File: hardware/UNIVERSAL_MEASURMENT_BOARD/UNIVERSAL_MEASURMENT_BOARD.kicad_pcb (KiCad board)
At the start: 2 copper layers, 180 parts, among them J1 2606-1110_010-000, J2 2606-1110_010-000, J28 FTSH-107-01-L-D-K, J3 2606-1110_010-000, J4 2606-1110_010-000, J5 2604-1104, U1 ADS8863IDGS, U10 TPS54202HDDCR, U11 CD4097BM, U12 TPS54202HDDCR, U13 L7805ABD2T-TR, U14 ADM3055EBRIZ-RL, U15 TLV76133KVUR, U16 TLV76133KVUR, U17 ESDS304DBVR, U18 ESDS304DBVR, U2 LT3471EDD#PBF, U3 MAX6063AEUR+T, U4 PGA280AIPW, U5 ISL21010CFH315Z-TK, U6 STM32G484RET3, U7 L7812ABD2T-TR, U8 MC7815BDTRKG, U9 MC79M15CDTRKG, Y1 ECS-1612MV

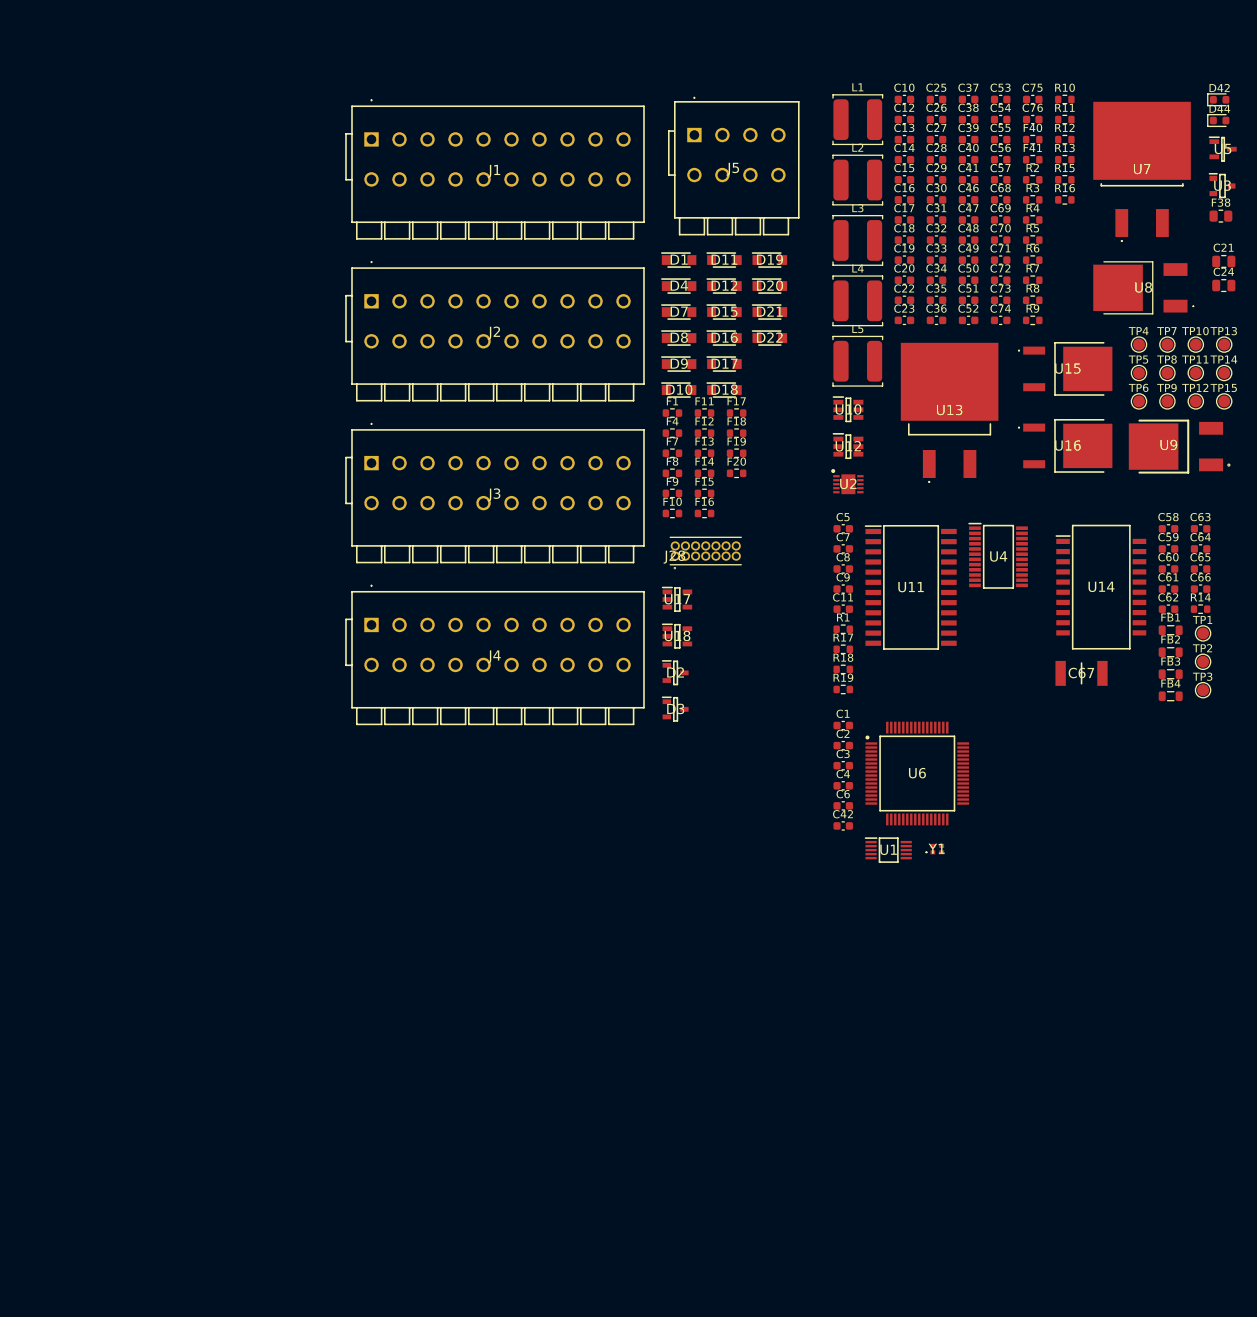
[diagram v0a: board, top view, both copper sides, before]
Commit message: first outcom of pcb design
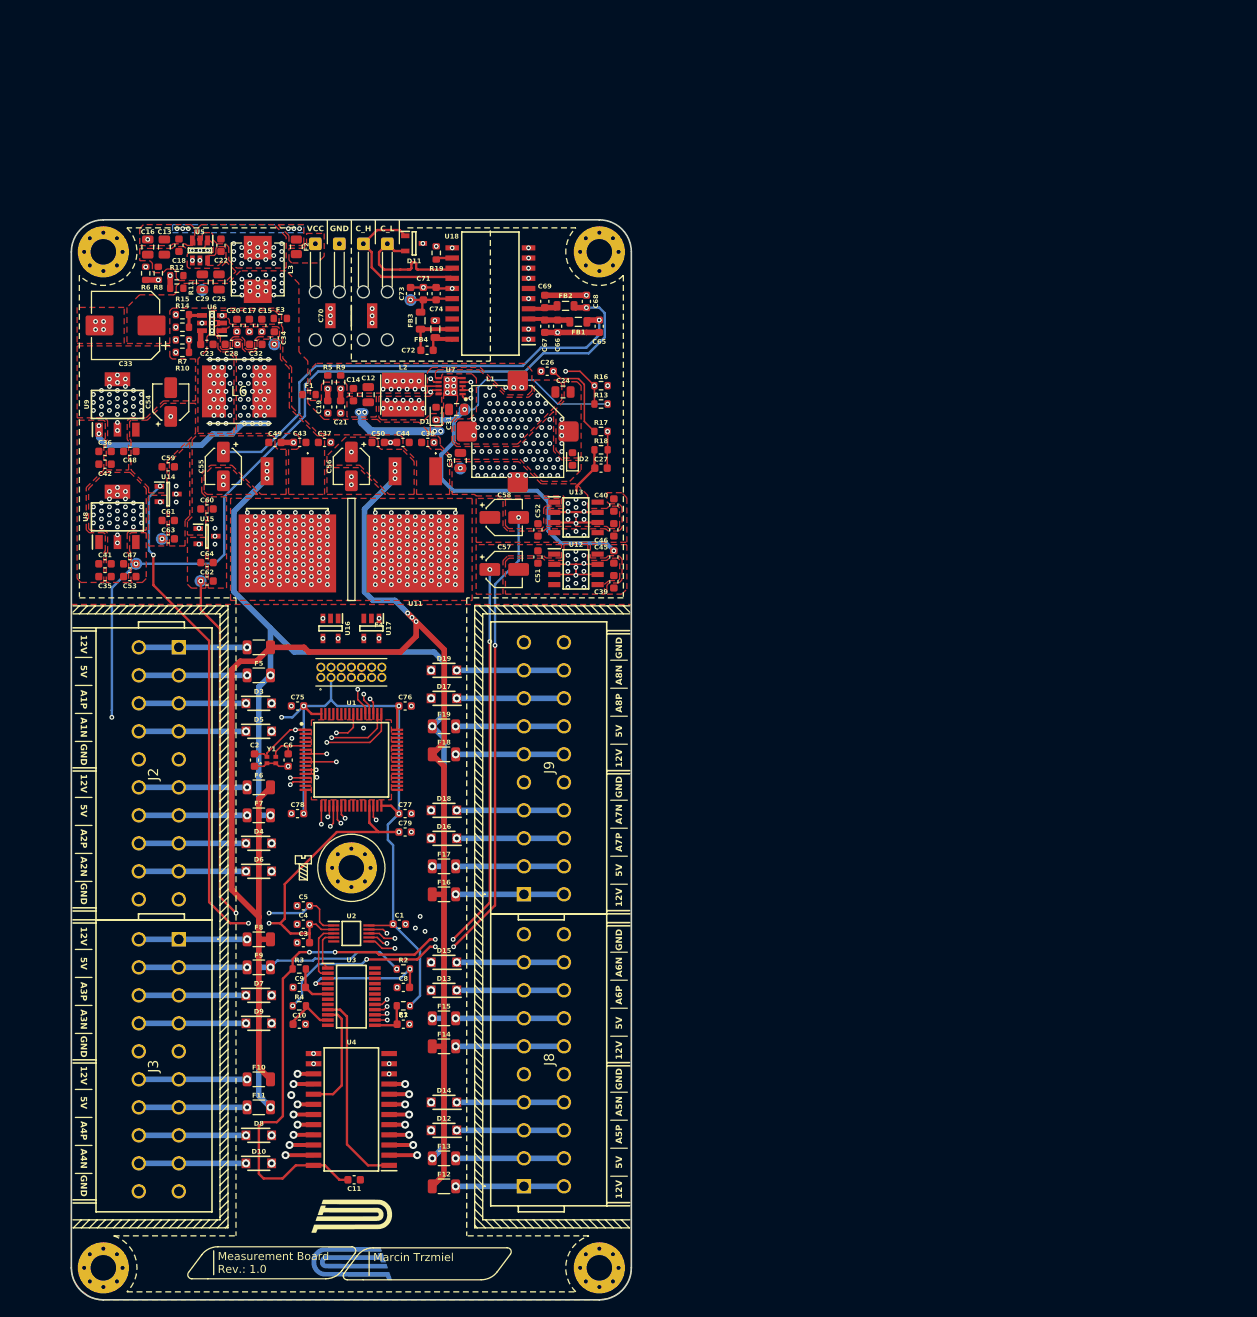
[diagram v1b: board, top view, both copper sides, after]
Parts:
- removed D20, D21, D22: ATV02W150-HF, ATV02W150-HF:SODFL3718X130N
- removed D42, D44: CDBU0340, Diode_SMD:D_0603_1608Metric
- removed F20: 100mA, Resistor_SMD:R_0603_1608Metric
- removed F38: 1,5A, Resistor_SMD:R_0805_2012Metric
- removed F40, F41: 300mA, Resistor_SMD:R_0603_1608Metric
- removed J28: FTSH-107-01-L-D-K, FTSH-107-01-L-D-K:FTSH-107-XX-YYY-D-K
- removed L4: 10uH, Inductor_SMD:L_TDK_VLS6045EX_VLS6045AF
- removed L5: 15uH, Inductor_SMD:L_TDK_VLS6045EX_VLS6045AF
- removed TP13: 3V3, TestPoint:TestPoint_Pad_D1.5mm
- removed TP14: 3V0A, TestPoint:TestPoint_Pad_D1.5mm
- removed the U4 at (182.1, 104.9)
- added C43: 330nF, REST:C_0603_1608Metric, F.Cu at (94.8, 90.6)
- added C44: 330nF, REST:C_0603_1608Metric, F.Cu at (107.7, 90.6)
- added C45: 330nF, REST:C_0603_1608Metric, F.Cu at (134.0, 104.9)
- added C77: 100nF, REST:C_0603_1608Metric, F.Cu at (107.9, 137.0)
- added C78: 100nF, REST:C_0603_1608Metric, F.Cu at (94.5, 137.0)
- added C79: 100nF, REST:C_0603_1608Metric, F.Cu at (107.9, 139.3)
- added D13: ATV02W150-HF, ATV02W150-HF:SODFL3718X130N, F.Cu at (112.8, 159.1)
- added D14: ATV02W150-HF, ATV02W150-HF:SODFL3718X130N, F.Cu at (112.8, 173.1)
- added D5: ATV02W150-HF, ATV02W150-HF:SODFL3718X130N, F.Cu at (89.7, 126.7)
- added D6: ATV02W150-HF, ATV02W150-HF:SODFL3718X130N, F.Cu at (89.7, 144.2)
- added F2: 1,5A, REST:F_0805_2012Metric, F.Cu at (94.3, 66.1)
- added F3: 300mA, REST:F_0603_1608Metric, F.Cu at (92.3, 75.1)
- added F5: 100mA, REST:F_1206_3216Metric, F.Cu at (89.7, 119.7)
- added F6: 100mA, REST:F_1206_3216Metric, F.Cu at (89.7, 133.7)
- added J6: Conn_01x01_Socket, REST:SolderWire-0.1sqmm_1x01_D0.4mm_OD1mm_Relief2x, F.Cu at (105.7, 65.8)
- added J7: Conn_01x01_Socket, REST:SolderWire-0.1sqmm_1x01_D0.4mm_OD1mm_Relief2x, F.Cu at (99.7, 65.8)
- added J8: 2606-1110_010-000, 2601-1110:26011110, F.Cu at (125.9, 167.7)
- added J9: 2606-1110_010-000, 2601-1110:26011110, F.Cu at (125.9, 131.2)
- added L6: ASPIAIG-S8050-221M-T, ASPIAIG-S8050-221M-T:INDPM8080X520N, F.Cu at (87.2, 84.2)
- added REF**: MountingHole_3.2mm_M3_Pad_Via, REST:MountingHole_3.2mm_M3_Pad_Via, F.Cu at (132.2, 193.8)
- added REF**: Screw_Generic_2.0x3.0mm_SilkScreen, Symbol:Screw_Generic_2.0x3.0mm_SilkScreen, F.Cu at (95.2, 143.8)
- added REF**: MountingHole_3.2mm_M3_Pad_Via, REST:MountingHole_3.2mm_M3_Pad_Via, F.Cu at (132.2, 66.8)
- added REF**: MountingHole_3.2mm_M3_Pad_Via, REST:MountingHole_3.2mm_M3_Pad_Via, F.Cu at (101.2, 143.8)
- added REF**: MountingHole_3.2mm_M3_Pad_Via, REST:MountingHole_3.2mm_M3_Pad_Via, F.Cu at (70.2, 193.8)
- added REF**: MountingHole_3.2mm_M3_Pad_Via, REST:MountingHole_3.2mm_M3_Pad_Via, F.Cu at (70.2, 66.8)
- added U11: L7812ABD2T-TR, L7812ABD2T-TR:L7812ABD2TTR, F.Cu at (109.2, 99.6)
- C1, C11, C19, C2, C22, C32, C38, C40, C49, C5, C6, C62, C75, C8, C9: footprint Capacitor_SMD:C_0603_1608Metric -> REST:C_0603_1608Metric
- C10: value 220uF -> 470nF; footprint Capacitor_SMD:C_0603_1608Metric -> REST:C_0603_1608Metric
- C12: value 1uF -> 10uF; footprint Capacitor_SMD:C_0603_1608Metric -> REST:C_0805_2012Metric
- C13: value 100nF -> 22uF; footprint Capacitor_SMD:C_0603_1608Metric -> REST:C_0805_2012Metric
- C14, C26, C47, C48, C50, C73, C76: value 22uF -> 100nF; footprint Capacitor_SMD:C_0603_1608Metric -> REST:C_0603_1608Metric
- C15: value 330nF -> 22uF; footprint Capacitor_SMD:C_0603_1608Metric -> REST:C_0603_1608Metric
- C16: value 220nF -> 22uF; footprint Capacitor_SMD:C_0603_1608Metric -> REST:C_0805_2012Metric
- C17, C35, C36, C39: value 1uF -> 22uF; footprint Capacitor_SMD:C_0603_1608Metric -> REST:C_0603_1608Metric
- C18, C68: value 10uF -> 100nF; footprint Capacitor_SMD:C_0603_1608Metric -> REST:C_0603_1608Metric
- C20, C23: value 1uF -> 100nF; footprint Capacitor_SMD:C_0603_1608Metric -> REST:C_0603_1608Metric
- C21: value 4.7uF -> 1uF; footprint Capacitor_SMD:C_0805_2012Metric -> REST:C_0603_1608Metric
- C24: value 10uF -> 1uF; footprint Capacitor_SMD:C_0805_2012Metric -> REST:C_0805_2012Metric
- C25: value 75pF -> 22uF; footprint Capacitor_SMD:C_0603_1608Metric -> REST:C_0805_2012Metric
- C27: value 330nF -> 75pF; footprint Capacitor_SMD:C_0603_1608Metric -> REST:C_0603_1608Metric
- C28: value 220nF -> 100nF; footprint Capacitor_SMD:C_0603_1608Metric -> REST:C_0603_1608Metric
- C29: value 1uF -> 22uF; footprint Capacitor_SMD:C_0603_1608Metric -> REST:C_0805_2012Metric
- C3: value 10nF -> 100nF; footprint Capacitor_SMD:C_0603_1608Metric -> REST:C_0603_1608Metric
- C30: value 100nF -> 10uF; footprint Capacitor_SMD:C_0603_1608Metric -> REST:C_0805_2012Metric
- C31: value 22uF -> 4.7uF; footprint Capacitor_SMD:C_0603_1608Metric -> REST:C_0805_2012Metric
- C33: value 100nF -> 220uF; footprint Capacitor_SMD:C_0603_1608Metric -> REST:CP_Elec_8x10
- C34, C37, C53: value 100nF -> 22uF; footprint Capacitor_SMD:C_0603_1608Metric -> REST:C_0603_1608Metric
- C4, C71: value 100nF -> 10nF; footprint Capacitor_SMD:C_0603_1608Metric -> REST:C_0603_1608Metric
- C41: value 22uF -> 330nF; footprint Capacitor_SMD:C_0603_1608Metric -> REST:C_0603_1608Metric
- C42, C46: value 100nF -> 330nF; footprint Capacitor_SMD:C_0603_1608Metric -> REST:C_0603_1608Metric
- C51: value 22uF -> 220nF; footprint Capacitor_SMD:C_0603_1608Metric -> REST:C_0603_1608Metric
- C52: value 330nF -> 220nF; footprint Capacitor_SMD:C_0603_1608Metric -> REST:C_0603_1608Metric
- C54: footprint Capacitor_SMD:C_0603_1608Metric -> REST:CP_Elec_4x5.8
- C55: value 22uF -> 10uF; footprint Capacitor_SMD:C_0603_1608Metric -> REST:CP_Elec_4x5.8
- C56: value 330nF -> 10uF; footprint Capacitor_SMD:C_0603_1608Metric -> REST:CP_Elec_4x5.8
- C57: value 100nF -> 1uF; footprint Capacitor_SMD:C_0603_1608Metric -> REST:CP_Elec_4x5.4
- C58: value 47uF -> 1uF; footprint Capacitor_SMD:C_0603_1608Metric -> REST:CP_Elec_4x5.4
- C59, C60: value 47uF -> 1uF; footprint Capacitor_SMD:C_0603_1608Metric -> REST:C_0603_1608Metric
- C61: value 47uF -> 100nF; footprint Capacitor_SMD:C_0603_1608Metric -> REST:C_0603_1608Metric
- C63: value 100nF -> 1uF; footprint Capacitor_SMD:C_0603_1608Metric -> REST:C_0603_1608Metric
- C64: value 10nF -> 1uF; footprint Capacitor_SMD:C_0603_1608Metric -> REST:C_0603_1608Metric
- C65: value 10nF -> 47uF; footprint Capacitor_SMD:C_0603_1608Metric -> REST:C_0603_1608Metric
- C66: value 100nF -> 47uF; footprint Capacitor_SMD:C_0603_1608Metric -> REST:C_0603_1608Metric
- C67: value 4.7nF/Y2 -> 100nF; footprint S252B222K502CT:CAPC5728X280N -> REST:C_0603_1608Metric
- C69: value 22uF -> 10nF; footprint Capacitor_SMD:C_0603_1608Metric -> REST:C_0603_1608Metric
- C7: value 470nF -> 100nF; footprint Capacitor_SMD:C_0603_1608Metric -> REST:C_0603_1608Metric
- C70: value 330nF -> 4.7nF/Y2; footprint Capacitor_SMD:C_0603_1608Metric -> S252B222K502CT:CAPC5728X280N
- C72: value 10uF -> 47uF; footprint Capacitor_SMD:C_0603_1608Metric -> REST:C_0603_1608Metric
- C74: value 330nF -> 47uF; footprint Capacitor_SMD:C_0603_1608Metric -> REST:C_0603_1608Metric
- D1: value ATV02W150-HF -> CDBU0340; footprint ATV02W150-HF:SODFL3718X130N -> REST:D_0603_1608Metric
- D11: value ATV02W150-HF -> PESD5V0L2BT,215; footprint ATV02W150-HF:SODFL3718X130N -> PESD5V0L2BT,215:SOT95P230X110-3N
- D2: value PESD5V0L2BT,215 -> CDBU0340; footprint PESD5V0L2BT,215:SOT95P230X110-3N -> REST:D_0603_1608Metric
- D3: value PESD5V0L2BT,215 -> ATV02W150-HF; footprint PESD5V0L2BT,215:SOT95P230X110-3N -> ATV02W150-HF:SODFL3718X130N
- F1: value 100mA -> 300mA; footprint Resistor_SMD:R_0603_1608Metric -> REST:F_0603_1608Metric
- F10, F11, F12, F13, F14, F15, F16, F17, F18, F19, F4, F7, F8, F9: footprint Resistor_SMD:R_0603_1608Metric -> REST:F_1206_3216Metric
- FB1, FB2, FB3, FB4: footprint Inductor_SMD:L_0805_2012Metric -> REST:L_0805_2012Metric
- J1: value 2606-1110_010-000 -> FTSH-107-01-L-D-K; footprint 2601-1110:26011110 -> FTSH-107-01-L-D-K:FTSH-107-XX-YYY-D-K
- J4: value 2606-1110_010-000 -> Conn_01x01_Socket; footprint 2601-1110:26011110 -> REST:SolderWire-0.1sqmm_1x01_D0.4mm_OD1mm_Relief2x
- J5: value 2604-1104 -> Conn_01x01_Socket; footprint 2601-1104:26011104 -> REST:SolderWire-0.1sqmm_1x01_D0.4mm_OD1mm_Relief2x
- L1: value 2.2uH -> PM3604-5-RC; footprint Inductor_SMD:L_TDK_VLS6045EX_VLS6045AF -> PM3604-5-RC:PM3604-5-RC
- L2: value 68uH/1.4A -> 74408943100; footprint Inductor_SMD:L_TDK_VLS6045EX_VLS6045AF -> 74408943100:WE-SPC_48XX78
- L3: value 68uH/1.4A -> 74437349560; footprint Inductor_SMD:L_TDK_VLS6045EX_VLS6045AF -> 74437349560:74437349560
- R1: value 22R -> 10R; footprint Resistor_SMD:R_0603_1608Metric -> REST:R_0603_1608Metric
- R10: value 649kR -> 73.2kR; footprint Resistor_SMD:R_0603_1608Metric -> REST:R_0603_1608Metric
- R11: footprint Resistor_SMD:R_0603_1608Metric -> REST:R_0603_1608Metric
- R12: value 64.9kR -> 10kR; footprint Resistor_SMD:R_0603_1608Metric -> REST:R_0603_1608Metric
- R13: value 10kR -> 255kR; footprint Resistor_SMD:R_0603_1608Metric -> REST:R_0603_1608Metric
- R14: value 100kR -> -R; footprint Resistor_SMD:R_0603_1608Metric -> REST:R_0603_1608Metric
- R15: value 15kR -> -R; footprint Resistor_SMD:R_0603_1608Metric -> REST:R_0603_1608Metric
- R16: value 274kR -> 15kR; footprint Resistor_SMD:R_0603_1608Metric -> REST:R_0603_1608Metric
- R17: value 22R -> 15kR; footprint Resistor_SMD:R_0603_1608Metric -> REST:R_0603_1608Metric
- R18: value 10R -> 274kR; footprint Resistor_SMD:R_0603_1608Metric -> REST:R_0603_1608Metric
- R19: value 10R -> 100kR; footprint Resistor_SMD:R_0603_1608Metric -> REST:R_0603_1608Metric
- R2: value 11kR -> 10R; footprint Resistor_SMD:R_0603_1608Metric -> REST:R_0603_1608Metric
- R3: value 11kR -> 22R; footprint Resistor_SMD:R_0603_1608Metric -> REST:R_0603_1608Metric
- R4: value 255kR -> 22R; footprint Resistor_SMD:R_0603_1608Metric -> REST:R_0603_1608Metric
- R5: value 15kR -> 11kR; footprint Resistor_SMD:R_0603_1608Metric -> REST:R_0603_1608Metric
- R6: value 681kR -> 649kR; footprint Resistor_SMD:R_0603_1608Metric -> REST:R_0603_1608Metric
- R7: value -R -> 681kR; footprint Resistor_SMD:R_0603_1608Metric -> REST:R_0603_1608Metric
- R8: value 73.2kR -> 64.9kR; footprint Resistor_SMD:R_0603_1608Metric -> REST:R_0603_1608Metric
- R9: value -R -> 11kR; footprint Resistor_SMD:R_0603_1608Metric -> REST:R_0603_1608Metric
- TP1: value C5V -> M15V; footprint TestPoint:TestPoint_Pad_D1.5mm -> REST:TestPoint_Pad_D1.5mm; moved to B.Cu
- TP10: value 12VA -> -15VA; footprint TestPoint:TestPoint_Pad_D1.5mm -> REST:TestPoint_Pad_D1.5mm; moved to B.Cu
- TP11: value 5VA -> 1V5A; footprint TestPoint:TestPoint_Pad_D1.5mm -> REST:TestPoint_Pad_D1.5mm; moved to B.Cu
- TP12: value 3V3A -> 3V0A; footprint TestPoint:TestPoint_Pad_D1.5mm -> REST:TestPoint_Pad_D1.5mm; moved to B.Cu
- TP15: value 1V5A -> CVISO; footprint TestPoint:TestPoint_Pad_D1.5mm -> REST:TestPoint_Pad_D1.5mm; moved to B.Cu
- TP2: value C3V -> -18V; footprint TestPoint:TestPoint_Pad_D1.5mm -> REST:TestPoint_Pad_D1.5mm; moved to B.Cu
- TP3: value CVISO -> 7V; footprint TestPoint:TestPoint_Pad_D1.5mm -> REST:TestPoint_Pad_D1.5mm; moved to B.Cu
- TP4: value M15V -> 18V; footprint TestPoint:TestPoint_Pad_D1.5mm -> REST:TestPoint_Pad_D1.5mm; moved to B.Cu
- TP5: value 18V -> 3V3; footprint TestPoint:TestPoint_Pad_D1.5mm -> REST:TestPoint_Pad_D1.5mm; moved to B.Cu
- TP6: value -18V -> 3V3A; footprint TestPoint:TestPoint_Pad_D1.5mm -> REST:TestPoint_Pad_D1.5mm; moved to B.Cu
- TP7: value 7V -> 5VA; footprint TestPoint:TestPoint_Pad_D1.5mm -> REST:TestPoint_Pad_D1.5mm; moved to B.Cu
- TP8: value 15VA -> 12VA; footprint TestPoint:TestPoint_Pad_D1.5mm -> REST:TestPoint_Pad_D1.5mm; moved to B.Cu
- TP9: value -15VA -> 15VA; footprint TestPoint:TestPoint_Pad_D1.5mm -> REST:TestPoint_Pad_D1.5mm; moved to B.Cu
- U1: value ADS8863IDGS -> STM32G484RET3; footprint ADS8863IDGS:SOP50P490X110-10N -> STM32G484RET3:QFP50P1200X1200X160-64N
- U10: value TPS54202HDDCR -> L7805ABD2T-TR; footprint TPS54202HDDCR:SOT95P280X110-6N -> L7805ABD2T-TR:L7805ABD2TTR
- U12: value TPS54202HDDCR -> L78L15ACD13TR; footprint TPS54202HDDCR:SOT95P280X110-6N -> LP358DR:SOIC127P600X175-8N
- U13: value L7805ABD2T-TR -> L79L15ACD13TR; footprint L7805ABD2T-TR:L7805ABD2TTR -> LP358DR:SOIC127P600X175-8N
- U14: value ADM3055EBRIZ-RL -> ISL21010CFH315Z-TK; footprint ADM3055EBRIZ-RL:SOIC127P1030X264-20N -> ISL21010CFH315Z-TK:SOT95P237X112-3N
- U15: value TLV76133KVUR -> ISL21010CFH330Z-TK; footprint TLV76133KVUR:TLV76133KVUR -> ISL21010CFH315Z-TK:SOT95P237X112-3N
- U16: value TLV76133KVUR -> ESDS304DBVR; footprint TLV76133KVUR:TLV76133KVUR -> ESDS304DBVR:SOT95P280X145-5N
- U18: value ESDS304DBVR -> ADM3055EBRIZ-RL; footprint ESDS304DBVR:SOT95P280X145-5N -> ADM3055EBRIZ-RL:SOIC127P1030X264-20N
- U2: value LT3471EDD#PBF -> ADS8863IDGS; footprint LT3471EDD#PBF:SON50P300X300X80-11N-D -> ADS8863IDGS:SOP50P490X110-10N
- U3: value MAX6063AEUR+T -> PGA280AIPW; footprint MAX6063AEUR+T:SOT95P229X119-3N -> PGA280AIPW:SOP65P640X120-24N
- U5: value ISL21010CFH315Z-TK -> TPS54202HDDCR; footprint ISL21010CFH315Z-TK:SOT95P237X112-3N -> TPS54202HDDCR:SOT95P280X110-6N
- U6: value STM32G484RET3 -> TPS54202HDDCR; footprint STM32G484RET3:QFP50P1200X1200X160-64N -> TPS54202HDDCR:SOT95P280X110-6N
- U7: value L7812ABD2T-TR -> LT3471EDD#PBF; footprint L7812ABD2T-TR:L7812ABD2TTR -> LT3471EDD#PBF:SON50P300X300X80-11N-D
- U8: value MC7815BDTRKG -> UA78M33CDCYRG3; footprint MC7815BDTRKG:NVD5117PLT4GVF01 -> UA78M33CDCYRG3:SOT230P700X180-4N
- U9: value MC79M15CDTRKG -> UA78M33CDCYRG3; footprint MC79M15CDTRKG:DPAK__SINGLE-GAUGE__TO-252_369C__ISSUE_F -> UA78M33CDCYRG3:SOT230P700X180-4N
- moved U3 148.7 mm to (101.2, 159.9)
- moved C10 138.1 mm to (94.7, 163.3)
- moved R4 134.4 mm to (94.7, 161.0)
- moved R3 132.8 mm to (94.7, 156.4)
- moved TP1 132.3 mm to (82.6, 71.5), turned to 180 degrees
- moved R14 132.1 mm to (80.1, 76.2), turned to 180 degrees
- moved TP11 130.9 mm to (77.5, 102.6), turned to 180 degrees
- moved C63 129.1 mm to (78.3, 102.6)
- moved U5 128.5 mm to (82.3, 66.6), turned to -90 degrees
- moved U9 127.9 mm to (72.0, 85.8), turned to 90 degrees
- moved TP5 127.6 mm to (74.3, 105.7), turned to 180 degrees
- moved U8 126.6 mm to (72.0, 99.9), turned to 90 degrees
- moved TP12 126.4 mm to (82.4, 107.9), turned to 180 degrees
- moved R2 126.2 mm to (107.7, 156.4)
- moved C59 125.5 mm to (78.3, 93.6)
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- renumbered U11 to U4
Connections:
- C10 pad 1: +15V0 -> Net-(U3-VSN)
- C11 pad 2: Net-(U4-DVDD) -> +15V0A
- C12 pad 1: +5V0A -> GND
- C12 pad 2: GND -> +15V0F
- C13 pad 2: +15V0F -> Net-(U5-VIN)
- C14 pad 1: +18V0 -> GND
- C14 pad 2: GND -> +15V0F
- C15 pad 1: +18V0 -> GND
- C15 pad 2: GND -> Net-(U6-VIN)
- C16 pad 1: +15V0A -> GND
- C16 pad 2: GND -> Net-(U5-VIN)
- C17 pad 1: +15V0A -> GND
- C17 pad 2: GND -> Net-(U6-VIN)
- C18 pad 2: +15V0F -> Net-(U5-VIN)
- C19 pad 2: Net-(U2-~{SHDN}/SS1) -> Net-(U7-~{SHDN}/SS1)
- C2 pad 1: +3V3A -> +3V3
- C20 pad 2: Net-(U2-~{SHDN}/SS2) -> Net-(U6-VIN)
- C21 pad 2: +18V0 -> Net-(U7-~{SHDN}/SS2)
- C22 pad 1: GND -> Net-(U5-BOOT)
- C22 pad 2: Net-(U2-FB1P) -> Net-(U5-SW)
- C23 pad 1: Net-(D44-A) -> Net-(U6-BOOT)
- C23 pad 2: Net-(U2-SW2) -> Net-(U6-SW)
- C24 pad 1: GND -> Net-(D2-A)
- C24 pad 2: -18V0 -> Net-(U7-SW2)
- C25 pad 1: -18V0 -> +15V0
- C25 pad 2: Net-(U2-FB2P) -> GND
- C26 pad 2: -18V0 -> Net-(U7-FB1P)
- C27 pad 1: GND -> -18V0
- C27 pad 2: -18V0 -> Net-(U7-FB2P)
- C28 pad 1: GND -> +7V0
- C28 pad 2: -15V0A -> GND
- C29 pad 1: GND -> +15V0
- C29 pad 2: -15V0A -> GND
- C30 pad 1: Net-(U10-BOOT) -> GND
- C30 pad 2: Net-(U10-SW) -> -18V0
- C31 pad 2: Net-(U10-VIN) -> +18V0
- C32 pad 1: GND -> +7V0
- C32 pad 2: Net-(U10-VIN) -> GND
- C33 pad 1: GND -> +15V0
- C33 pad 2: Net-(U10-VIN) -> GND
- C34 pad 1: +1V5A -> +7V0
- C35 pad 1: +1V5A -> +7V0
- C36 pad 1: +3V3A -> +7V0
- C37 pad 1: +3V0A -> +7V0
- C38 pad 1: +7V0 -> +15V0
- C39 pad 1: +3V0A -> +18V0
- C4 pad 1: +3V0A -> +3V3A
- C40 pad 1: +15V0 -> GND
- C40 pad 2: GND -> -18V0
- C42 pad 1: +3V3 -> +7V0
- C46 pad 1: Net-(U12-BOOT) -> GND
- C46 pad 2: Net-(U12-SW) -> -18V0
- C47 pad 1: GND -> +3V3
- C47 pad 2: Net-(U12-VIN) -> GND
- C48 pad 1: GND -> +3V3A
- C48 pad 2: Net-(U12-VIN) -> GND
- C49 pad 1: GND -> +5V0A
- C49 pad 2: Net-(U12-VIN) -> GND
- C5 pad 1: GND -> +3V0A
- C5 pad 2: +15V0A -> GND
- C50 pad 1: +15V0 -> +12V0A
- C51 pad 1: +15V0 -> +15V0A
- C52 pad 1: +15V0 -> GND
- C52 pad 2: GND -> -15V0A
- C53 pad 1: +12V0A -> +3V3
- C54 pad 1: +12V0A -> +3V3A
- C55 pad 1: +7V0 -> +5V0A
- C56 pad 1: +7V0 -> +12V0A
- C57 pad 1: +5V0A -> +15V0A
- C58 pad 1: Net-(U14-VISOOUT) -> GND
- C58 pad 2: Net-(U14-GNDISO) -> -15V0A
- C59 pad 1: VISO -> +3V3A
- C59 pad 2: BUS_GND -> GND
- C61 pad 1: Net-(U14-VCC) -> +1V5A
- C62 pad 1: Net-(U14-VCC) -> +3V0A
- C63 pad 1: +3V3 -> +1V5A
- C64 pad 1: Net-(U14-VIO) -> +3V0A
- C65 pad 1: VISO -> +5V0A
- C65 pad 2: BUS_GND -> GND
- C66 pad 1: VISO -> Net-(U18-VCC)
- C66 pad 2: BUS_GND -> GND
- C67 pad 1: BUS_GND -> Net-(U18-VCC)
- C68 pad 1: +5V0A -> +3V3
- C69 pad 1: +7V0 -> Net-(U18-VIO)
- C7 pad 2: Net-(U4-VSP) -> Net-(U3-DVDD)
- C70 pad 1: +7V0 -> GND_ISO
- C71 pad 1: +3V3A -> VISO
- C71 pad 2: GND -> GND_ISO
- C72 pad 1: +3V3A -> Net-(U18-VISOOUT)
- C72 pad 2: GND -> Net-(U18-GNDISO)
- C73 pad 1: +7V0 -> VISO
- C73 pad 2: GND -> GND_ISO
- C74 pad 1: +7V0 -> VISO
- C74 pad 2: GND -> GND_ISO
- C8 pad 1: Net-(U4-VSN) -> GND
- C8 pad 2: GND -> Net-(U3-VSOP)
- C9 pad 2: Net-(U4-VSOP) -> Net-(U3-VSP)
- D1 pad 1: /connectors/A1P -> +18V0
- D1 pad 2: GND -> Net-(D1-A)
- D10 pad 1: /connectors/A3N -> /connectors/A4N
- D11 pad 1: /connectors/A4P -> /can/CANH
- D11 pad 2: GND -> /can/CANL
- D12 pad 1: /connectors/A4N -> /connectors/A5P
- D15 pad 1: /connectors/A5P -> /connectors/A6N
- D16 pad 1: /connectors/A5N -> /connectors/A7P
- D17 pad 1: /connectors/A6P -> /connectors/A8P
- D18 pad 1: /connectors/A6N -> /connectors/A7N
- D19 pad 1: /connectors/A7P -> /connectors/A8N
- D2 pad 1: /can/CANL -> GND
- D2 pad 2: (no net) -> Net-(D2-A)
- D3 pad 1: (no net) -> /connectors/A1P
- D3 pad 2: /can/CANH -> GND
- D4 pad 1: /connectors/A1N -> /connectors/A2P
- D7 pad 1: /connectors/A2P -> /connectors/A3P
- D8 pad 1: /connectors/A2N -> /connectors/A4P
- D9 pad 1: /connectors/A3P -> /connectors/A3N
- F1 pad 1: +12V0 -> +15V0
- F1 pad 2: Net-(F1-Pad2) -> +15V0F
- F10 pad 1: +5V0 -> +12V0A
- F11 pad 1: +12V0 -> +5V0A
- F12 pad 1: +5V0 -> +12V0A
- F13 pad 1: +12V0 -> +5V0A
- F14 pad 1: +5V0 -> +12V0A
- F15 pad 1: +12V0 -> +5V0A
- F16 pad 1: +5V0 -> +12V0A
- F17 pad 1: +12V0 -> +5V0A
- F18 pad 1: +5V0 -> +12V0A
- F19 pad 1: +12V0 -> +5V0A
- F4 pad 1: +5V0 -> +12V0A
- F7 pad 1: +12V0 -> +5V0A
- F8 pad 1: +12V0 -> +12V0A
- F9 pad 1: +5V0 -> +5V0A
- FB1 pad 1: Net-(U14-VCC) -> Net-(U18-VCC)
- FB2 pad 1: VISO -> Net-(U18-VIO)
- FB2 pad 2: Net-(U14-VISOOUT) -> +3V3
- FB3 pad 1: Net-(U14-VIO) -> VISO
- FB3 pad 2: +3V3 -> Net-(U18-VISOOUT)
- FB4 pad 1: BUS_GND -> GND_ISO
- FB4 pad 2: Net-(U14-GNDISO) -> Net-(U18-GNDISO)
- J1 pad 1: Net-(F1-Pad2) -> unconnected-(J1-Pin_1-Pad1)
- J1 pad 10: GND -> unconnected-(J1-Pin_10-Pad10)
- J1 pad 11: (no net) -> GND
- J1 pad 12: (no net) -> /connectors/NRST
- J1 pad 13: (no net) -> /connectors/UART_RX_PROG
- J1 pad 14: (no net) -> /connectors/UART_TX_PROG
- J1 pad 2: Net-(F4-Pad2) -> unconnected-(J1-Pin_2-Pad2)
- J1 pad 3: /connectors/A1P -> +3V3
- J1 pad 4: /connectors/A1N -> /connectors/SWDIO
- J1 pad 6: Net-(F7-Pad2) -> /connectors/SWCLK
- J1 pad 7: Net-(F10-Pad2) -> GND
- J1 pad 8: /connectors/A2P -> /connectors/SWO
- J1 pad 9: /connectors/A2N -> unconnected-(J1-Pin_9-Pad9)
- J2 pad 1: Net-(F8-Pad2) -> Net-(F4-Pad2)
- J2 pad 2: Net-(F9-Pad2) -> Net-(F5-Pad2)
- J2 pad 3: /connectors/A3P -> /connectors/A1P
- J2 pad 4: /connectors/A3N -> /connectors/A1N
- J2 pad 6: Net-(F11-Pad2) -> Net-(F6-Pad2)
- J2 pad 7: Net-(F12-Pad2) -> Net-(F7-Pad2)
- J2 pad 8: /connectors/A4P -> /connectors/A2P
- J2 pad 9: /connectors/A4N -> /connectors/A2N
- J3 pad 1: Net-(F13-Pad2) -> Net-(F8-Pad2)
- J3 pad 2: Net-(F14-Pad2) -> Net-(F9-Pad2)
- J3 pad 3: /connectors/A5P -> /connectors/A3P
- J3 pad 4: /connectors/A5N -> /connectors/A3N
- J3 pad 6: Net-(F15-Pad2) -> Net-(F10-Pad2)
- J3 pad 7: Net-(F16-Pad2) -> Net-(F11-Pad2)
- J3 pad 8: /connectors/A6P -> /connectors/A4P
- J3 pad 9: /connectors/A6N -> /connectors/A4N
- J4 pad 1: Net-(F17-Pad2) -> +24V0
- J5 pad 1: +24V0 -> /can/CANH
- L1 pad 2: Net-(D42-A) -> Net-(U7-SW2)
- L2 pad 1: Net-(U10-SW) -> +15V0F
- L2 pad 2: +7V0 -> Net-(D1-A)
- L3 pad 1: Net-(U12-SW) -> Net-(U5-SW)
- R1 pad 1: -15V0A -> +3V3
- R1 pad 2: Net-(U4-VSN) -> Net-(U3-DVDD)
- R10 pad 1: Net-(U12-VIN) -> GND
- R10 pad 2: Net-(U12-EN) -> Net-(U6-EN)
- R11 pad 1: Net-(U12-FB) -> Net-(U5-FB)
- R12 pad 2: Net-(U12-EN) -> Net-(U5-FB)
- R13 pad 1: GND -> Net-(U7-FB1N)
- R13 pad 2: Net-(U12-FB) -> +18V0
- R14 pad 1: Net-(U14-RS) -> Net-(U6-FB)
- R14 pad 2: BUS_GND -> +7V0
- R15 pad 1: Net-(U2-FB2P) -> GND
- R15 pad 2: Net-(U2-FB1P) -> Net-(U6-FB)
- R16 pad 1: -18V0 -> Net-(U7-FB1N)
- R16 pad 2: Net-(U2-FB2P) -> GND
- R17 pad 1: +15V0A -> Net-(U7-FB2P)
- R17 pad 2: Net-(U4-VSP) -> Net-(U7-FB1P)
- R18 pad 1: +5V0A -> -18V0
- R18 pad 2: Net-(U4-VSOP) -> Net-(U7-FB2P)
- R19 pad 1: +3V3 -> Net-(U18-RS)
- R19 pad 2: Net-(U4-DVDD) -> GND_ISO
- R2 pad 1: +15V0F -> +5V0A
- R2 pad 2: Net-(U2-~{SHDN}/SS1) -> Net-(U3-VSOP)
- R3 pad 1: +15V0F -> +15V0A
- R3 pad 2: Net-(U2-~{SHDN}/SS2) -> Net-(U3-VSP)
- R4 pad 1: Net-(U2-FB1N) -> -15V0A
- R4 pad 2: +18V0 -> Net-(U3-VSN)
- R5 pad 1: Net-(U2-FB1N) -> +15V0F
- R5 pad 2: GND -> Net-(U7-~{SHDN}/SS1)
- R6 pad 1: Net-(U10-VIN) -> Net-(U5-VIN)
- R6 pad 2: Net-(U10-EN) -> Net-(U5-EN)
- R7 pad 1: Net-(U10-FB) -> Net-(U6-VIN)
- R7 pad 2: +7V0 -> Net-(U6-EN)
- R8 pad 2: Net-(U10-EN) -> Net-(U5-EN)
- R9 pad 1: GND -> +15V0F
- R9 pad 2: Net-(U10-FB) -> Net-(U7-~{SHDN}/SS2)
- TP1 pad 1: Net-(U14-VCC) -> +15V0
- TP10 pad 1: +12V0A -> -15V0A
- TP11 pad 1: +5V0A -> +1V5A
- TP12 pad 1: +3V3A -> +3V0A
- TP15 pad 1: +1V5A -> VISO
- TP2 pad 1: Net-(U14-VIO) -> -18V0
- TP3 pad 1: VISO -> +7V0
- TP4 pad 1: +15V0 -> +18V0
- TP5 pad 1: +18V0 -> +3V3
- TP6 pad 1: -18V0 -> +3V3A
- TP7 pad 1: +7V0 -> +5V0A
- TP8 pad 1: +15V0A -> +12V0A
- TP9 pad 1: -15V0A -> +15V0A
- U1 pad 1: +3V0A -> +3V3
- U1 pad 10: +3V3 -> unconnected-(U1-PC2-Pad10)
- U1 pad 2: +3V3A -> unconnected-(U1-PC13-Pad2)
- U1 pad 3: /mcu & adc/AINP -> unconnected-(U1-PC14-Pad3)
- U1 pad 4: /mcu & adc/AINN -> unconnected-(U1-PC15-Pad4)
- U1 pad 5: GND -> /mcu & adc/HSE
- U1 pad 6: /mcu & adc/ADCCS -> unconnected-(U1-PF1-Pad6)
- U1 pad 7: /mcu & adc/MOSI -> /connectors/NRST
- U1 pad 8: /mcu & adc/SCLK -> unconnected-(U1-PC0-Pad8)
- U1 pad 9: /mcu & adc/MISO -> /connectors/UART_TX_PROG
- U10 pad 1: GND -> +7V0
- U10 pad 2: Net-(U10-SW) -> GND
- U10 pad 3: Net-(U10-VIN) -> +5V0A
- U12 pad 1: GND -> +15V0A
- U12 pad 2: Net-(U12-SW) -> GND
- U12 pad 3: Net-(U12-VIN) -> GND
- U12 pad 4: Net-(U12-FB) -> Net-(U12-NC_1)
- U12 pad 5: Net-(U12-EN) -> Net-(U12-NC_1)
- U12 pad 6: Net-(U12-BOOT) -> GND
- U13 pad 1: +7V0 -> -15V0A
- U13 pad 2: GND -> -18V0
- U13 pad 3: +5V0A -> -18V0
- U14 pad 1: GND -> +3V3A
- U14 pad 2: GND -> +1V5A
- U14 pad 3: Net-(U14-VCC) -> GND
- U15 pad 1: GND -> +5V0A
- U15 pad 2: +3V3A -> +3V0A
- U15 pad 3: +7V0 -> GND
- U16 pad 1: GND -> unconnected-(U16-Pad1)
- U16 pad 2: +3V3 -> GND
- U16 pad 3: +7V0 -> /connectors/SWDIO
- U17 pad 1: /connectors/NRST -> /connectors/UART_RX_PROG
- U17 pad 3: /connectors/SWO -> unconnected-(U17-Pad3)
- U17 pad 4: /connectors/SWCLK -> /connectors/NRST
- U17 pad 5: /connectors/SWDIO -> /connectors/UART_TX_PROG
- U18 pad 1: +3.3V -> GND
- U18 pad 3: unconnected-(U18-Pad3) -> Net-(U18-VCC)
- U18 pad 4: /connectors/UART_TX_PROG -> Net-(U18-VIO)
- U18 pad 5: /connectors/UART_RX_PROG -> /can/CAN_RX
- U2 pad 1: Net-(U2-FB1N) -> +3V0A
- U2 pad 10: Net-(D42-A) -> +3V3
- U2 pad 2: Net-(U2-FB1P) -> +3V3A
- U2 pad 3: Net-(U2-FB1P) -> /mcu & adc/AINP
- U2 pad 4: Net-(U2-FB2P) -> /mcu & adc/AINN
- U2 pad 6: Net-(U2-SW2) -> /mcu & adc/ADCCS
- U2 pad 7: Net-(U2-~{SHDN}/SS2) -> /mcu & adc/MOSI
- U2 pad 8: +15V0F -> /mcu & adc/SCLK
- U2 pad 9: Net-(U2-~{SHDN}/SS1) -> /mcu & adc/MISO
- U3 pad 1: +5V0A -> /mcu & adc/AINN
- U3 pad 2: +3V0A -> /mcu & adc/AINP
- U3 pad 3: GND -> 1V5A
- U5 pad 1: +3V3A -> GND
- U5 pad 2: +1V5A -> Net-(U5-SW)
- U5 pad 3: GND -> Net-(U5-VIN)
- U6 pad 1: +3V3 -> GND
- U6 pad 2: unconnected-(U6-PC13-Pad2) -> Net-(U6-SW)
- U6 pad 3: unconnected-(U6-PC14-Pad3) -> Net-(U6-VIN)
- U6 pad 4: unconnected-(U6-PC15-Pad4) -> Net-(U6-FB)
- U6 pad 5: /mcu & adc/HSE -> Net-(U6-EN)
- U6 pad 6: unconnected-(U6-PF1-Pad6) -> Net-(U6-BOOT)
- U7 pad 1: +15V0 -> Net-(U7-FB1N)
- U7 pad 2: GND -> Net-(U7-FB1P)
- U7 pad 3: +12V0A -> Net-(U7-FB1P)
- U8 pad 1: +18V0 -> +7V0
- U8 pad 3: +15V0A -> +3V3
- U9 pad 1: GND -> +7V0
- U9 pad 2: -15V0A -> GND
- U9 pad 3: -18V0 -> +3V3A
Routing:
- net +5V0A: track 0.00 -> 254.7 mm, vias 0 -> 15
- net +3V3: track 0.00 -> 221.8 mm, vias 0 -> 11
- net +12V0A: track 0.00 -> 202.4 mm, vias 0 -> 7
- net /connectors/A8N: track 0.00 -> 118.8 mm, vias 0 -> 2
- net +15V0A: track 0.00 -> 111.8 mm, vias 0 -> 6
- net /connectors/A1P: track 0.00 -> 108.5 mm, vias 0 -> 2
- net /connectors/A7N: track 0.00 -> 103.9 mm, vias 0 -> 2
- net +3V3A: track 0.00 -> 101.3 mm, vias 0 -> 7
- net /connectors/A8P: track 0.00 -> 94.3 mm, vias 0 -> 2
- net /connectors/A2P: track 0.00 -> 93.6 mm, vias 0 -> 2
- net /connectors/A6N: track 0.00 -> 84.9 mm, vias 0 -> 2
- net /connectors/A1N: track 0.00 -> 84.5 mm, vias 0 -> 2
- net /connectors/A7P: track 0.00 -> 81.9 mm, vias 0 -> 2
- net -15V0A: track 0.00 -> 81.4 mm, vias 0 -> 6
- net /can/CAN_STB: track 0.00 -> 76.1 mm, vias 0 -> 2
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- added copper zone on F.Cu, net +12V0A
- added copper zone on F.Cu, net +15V0
- added copper zone on F.Cu, net +15V0A
- added copper zone on F.Cu, net +15V0F
- added copper zone on F.Cu, net +18V0
- added copper zone on F.Cu, net +1V5A
- added copper zone on F.Cu, net +24V0
- added copper zone on F.Cu, net +3V0A
- added copper zone on F.Cu, net +3V3
- added copper zone on F.Cu, net +3V3A
- added copper zone on F.Cu, net +5V0A
- added copper zone on F.Cu, net +7V0
- added copper zone on F.Cu, net -15V0A
- added copper zone on F.Cu, net -18V0
- added copper zone on F.Cu, net GND
- added copper zone on In1.Cu, net GND
- added copper zone on In4.Cu, net GND
- added copper zone on In1.Cu, net GND_ISO
- added copper zone on F.Cu, net Net-(D1-A)
- added copper zone on F.Cu, net Net-(D2-A)
- added copper zone on F.Cu, net Net-(U5-BOOT)
- added copper zone on F.Cu, net Net-(U5-SW)
- added copper zone on B.Cu, net Net-(U5-VIN)
- added copper zone on F.Cu, net Net-(U5-VIN)
- added copper zone on F.Cu, net Net-(U6-SW)
- added copper zone on F.Cu, net Net-(U6-VIN)
- added copper zone on F.Cu, net Net-(U7-SW2)
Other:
- board outline added: 70 x 135 mm
- copper layers 2 -> 6
- board text added: "12V"
- board text added: "5V"
- board text added: "A1N"
- board text added: "A1P"
- board text added: "A2N"
- board text added: "A2P"
- board text added: "A3N"
- board text added: "A3P"
- board text added: "A4N"
- board text added: "A4P"
- board text added: "A5N"
- board text added: "A5P"
- board text added: "A6N"
- board text added: "A6P"
- board text added: "A7N"
- board text added: "A7P"
- board text added: "A8N"
- board text added: "A8P"
- board text added: "C40"
- board text added: "C45"
- board text added: "C51"
- board text added: "C_H"
- board text added: "C_L"
- board text added: "GND"
- board text added: "ISOLATED"
- board text added: "Marcin Trzmiel"
- board text added: "Measurement Board Rev.: 1.0"
- board text added: "STACKUP: 1. SIGNAL / POWER 2. GND 3. SIGNAL 4. SIGNAL 5. GND 6. SIGNAL / POWER"
- board text added: "U10"
- board text added: "U12"
- board text added: "U9"
- board text added: "VCC"

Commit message: Review fixes
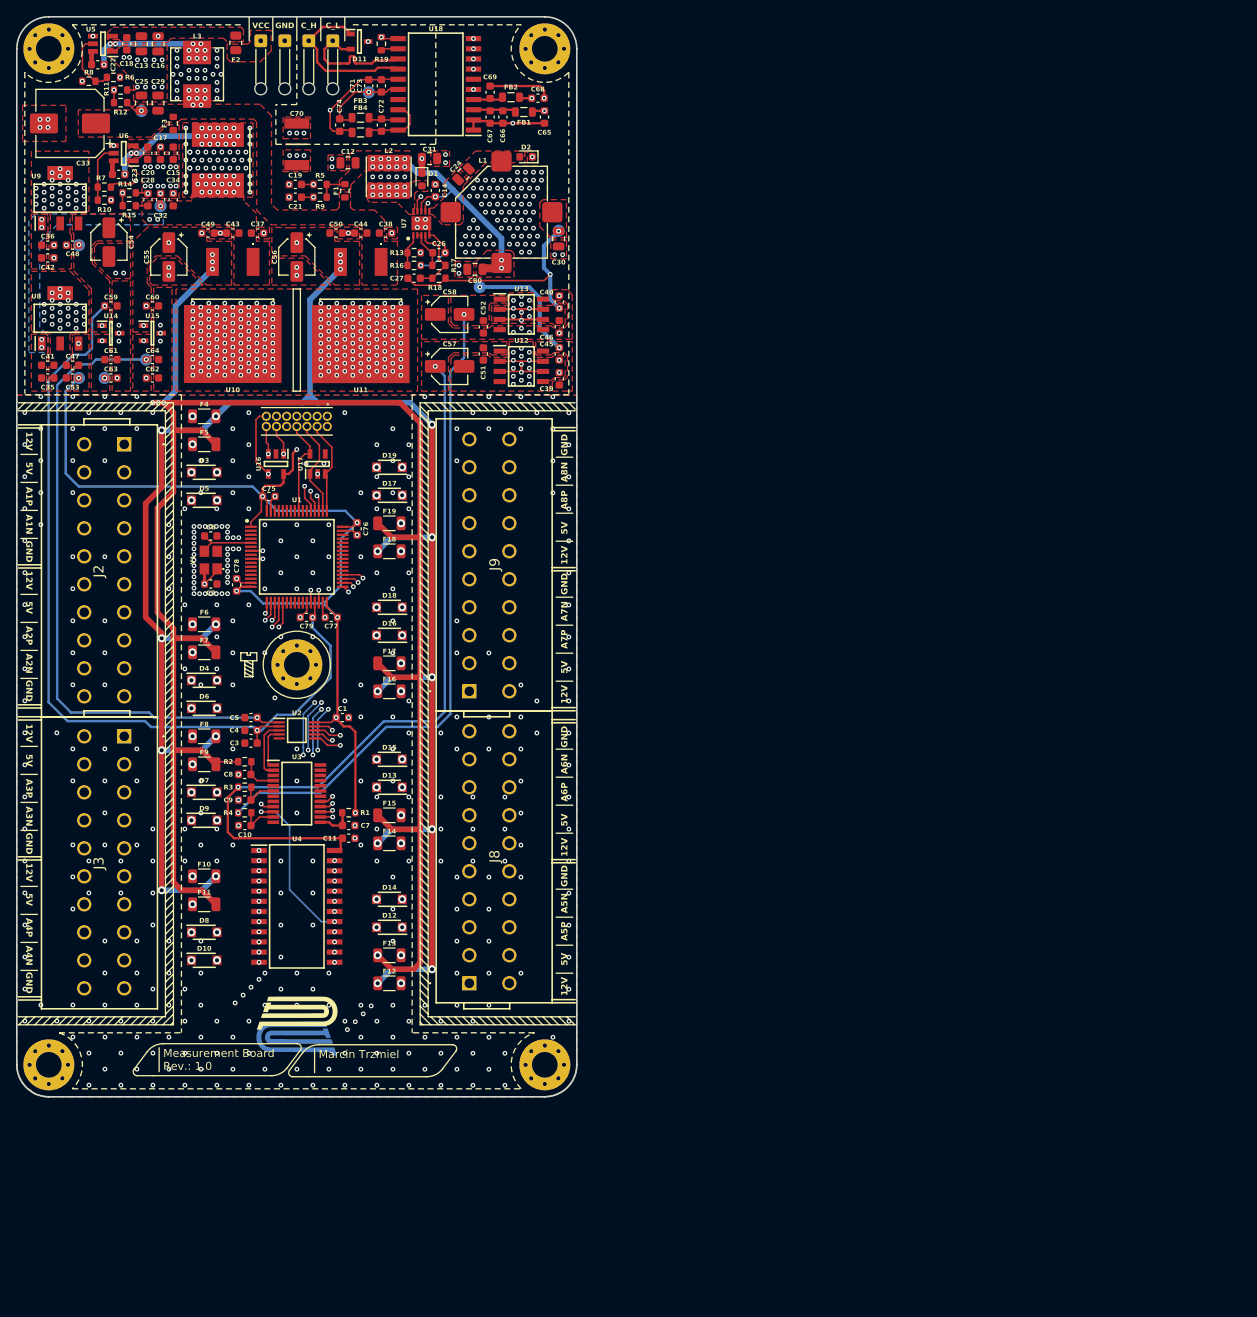
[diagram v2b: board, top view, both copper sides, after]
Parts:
- added C80: 10uF, REST:C_0805_2012Metric, F.Cu at (116.7, 68.9)
- J4, J5, J6, J7: footprint REST:SolderWire-0.1sqmm_1x01_D0.4mm_OD1mm_Relief2x -> REST:SolderPoint
- U18: value ADM3055EBRIZ-RL -> ADM3057EBRWZ; footprint ADM3055EBRIZ-RL:SOIC127P1030X264-20N -> ADM3057EBRWZ:SOIC127P1032X265-20N
- Y1: value ECS-1612MV -> ATX-H11-F-16.000MHz-G100-T; footprint ECS-1612MV-080-CN-TR:ECS1612MV080CNTR -> ATX-H11-F-16.000MHz-G100-T:ATXH11F16000MHzG100T
- moved C11 42.7 mm to (100.9, 140.1)
- moved D2 38.2 mm to (123.1, 54.9), turned to 180 degrees
- moved C27 33.3 mm to (109.1, 70.0)
- moved C8 33.2 mm to (87.9, 132.1)
- moved R2 32.6 mm to (87.9, 130.5)
- moved TP2 32.2 mm to (127.1, 64.1)
- moved J1 32.1 mm to (94.4, 87.9), turned to 180 degrees
- moved C31 31.5 mm to (111.0, 55.1), turned to 180 degrees
- moved C30 30.3 mm to (127.1, 65.1), turned to 90 degrees
- moved R13 30.1 mm to (109.1, 66.9)
- moved C24 29.9 mm to (115.2, 57.1), turned to -135 degrees
- moved D3 29.7 mm to (82.8, 94.3)
- moved D5 29.7 mm to (82.8, 97.8)
- moved F4 29.7 mm to (82.8, 87.3)
- moved F5 29.7 mm to (82.8, 90.8)
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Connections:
- L1 pad 1: +15V0F -> Net-(U7-SW2)
- L1 pad 2: Net-(U7-SW2) -> +15V0F
- U1 pad 11: /mcu & adc/ADDR2 -> unconnected-(U1-PC3-Pad11)
- U1 pad 12: /mcu & adc/ADDR1 -> unconnected-(U1-PA0-Pad12)
- U1 pad 13: /mcu & adc/MUXEN -> unconnected-(U1-PA1-Pad13)
- U1 pad 14: /mcu & adc/ADDR3 -> unconnected-(U1-PA2-Pad14)
- U1 pad 18: unconnected-(U1-PA4-Pad18) -> /mcu & adc/ADCCS
- U1 pad 22: /mcu & adc/ADCCS -> unconnected-(U1-PC4-Pad22)
- U1 pad 33: unconnected-(U1-PB11-Pad33) -> /mcu & adc/ADDR1
- U1 pad 34: unconnected-(U1-PB12-Pad34) -> /mcu & adc/ADDR2
- U1 pad 35: unconnected-(U1-PB13-Pad35) -> /mcu & adc/MUXEN
- U1 pad 36: unconnected-(U1-PB14-Pad36) -> /mcu & adc/ADDR3
- U16 pad 1: unconnected-(U16-Pad1) -> /connectors/NRST
- U16 pad 3: /connectors/SWDIO -> /connectors/UART_TX_PROG
- U16 pad 4: /connectors/SWCLK -> /connectors/UART_RX_PROG
- U16 pad 5: /connectors/SWO -> +3V3
- U17 pad 1: /connectors/UART_RX_PROG -> /connectors/SWCLK
- U17 pad 3: unconnected-(U17-Pad3) -> /connectors/SWDIO
- U17 pad 4: /connectors/NRST -> GND
- U17 pad 5: /connectors/UART_TX_PROG -> /connectors/SWO
- Y1 pad 1: GND -> +3V3
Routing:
- net /connectors/A1N: track 84.5 -> 139.4 mm
- net /connectors/A8P: track 94.3 -> 144.2 mm, vias 2 -> 3
- net /connectors/A2N: track 71.8 -> 117.2 mm
- net +5V0A: track 254.7 -> 299.7 mm, vias 15 -> 12
- net /connectors/A7P: track 81.9 -> 121.0 mm, vias 2 -> 3
- net +12V0A: track 202.4 -> 236.1 mm, vias 7 -> 21
- net /connectors/A3N: track 57.8 -> 90.8 mm
- net +7V0: track 33.1 -> 1.84 mm, vias 41 -> 23
- net /connectors/A6P: track 67.6 -> 96.8 mm, vias 2 -> 3
- net +15V0F: track 5.17 -> 32.7 mm, vias 14 -> 13
- net /connectors/SWDIO: track 36.1 -> 11.7 mm, vias 2 -> 0
- net -18V0: track 29.9 -> 53.1 mm, vias 24 -> 13
- net /connectors/A4N: track 45.0 -> 67.9 mm
- net +3V0A: track 57.9 -> 80.6 mm, vias 5 -> 4
- net +18V0: track 61.5 -> 41.8 mm
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- added copper zone on B.Cu, net +7V0
- added copper zone on B.Cu, net GND
- added copper zone on In2.Cu, net GND
- added copper zone on In3.Cu, net GND
- added copper zone on F.Cu, net GND_ISO
- removed copper zone on F.Cu, net Net-(U5-BOOT)
- removed copper zone on F.Cu, net Net-(U5-SW)
- removed copper zone on B.Cu, net Net-(U5-VIN)
- removed copper zone on F.Cu, net Net-(U6-SW)
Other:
- board text added: "L6"
- board text added: "STACKUP: 1. SIGNAL / POWER 2. GND 3. SIGNAL / POWER ON PS 4. SIGNAL / POWER ON PS 5. GND 6. SIGNAL / POWER"
- board text removed: "STACKUP: 1. SIGNAL / POWER 2. GND 3. SIGNAL 4. SIGNAL 5. GND 6. SIGNAL / POWER"
